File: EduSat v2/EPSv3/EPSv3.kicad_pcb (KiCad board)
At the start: 2 copper layers, 1 part

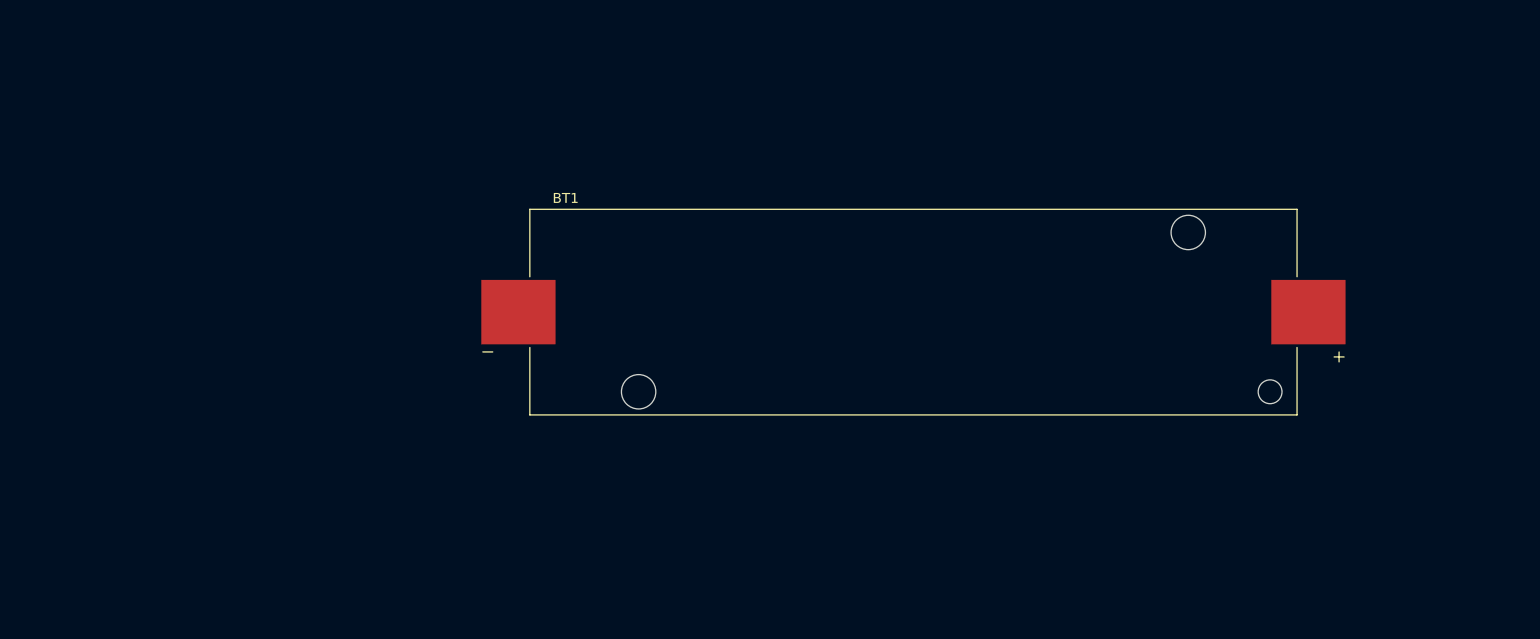
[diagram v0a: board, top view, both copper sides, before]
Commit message: EPS updates
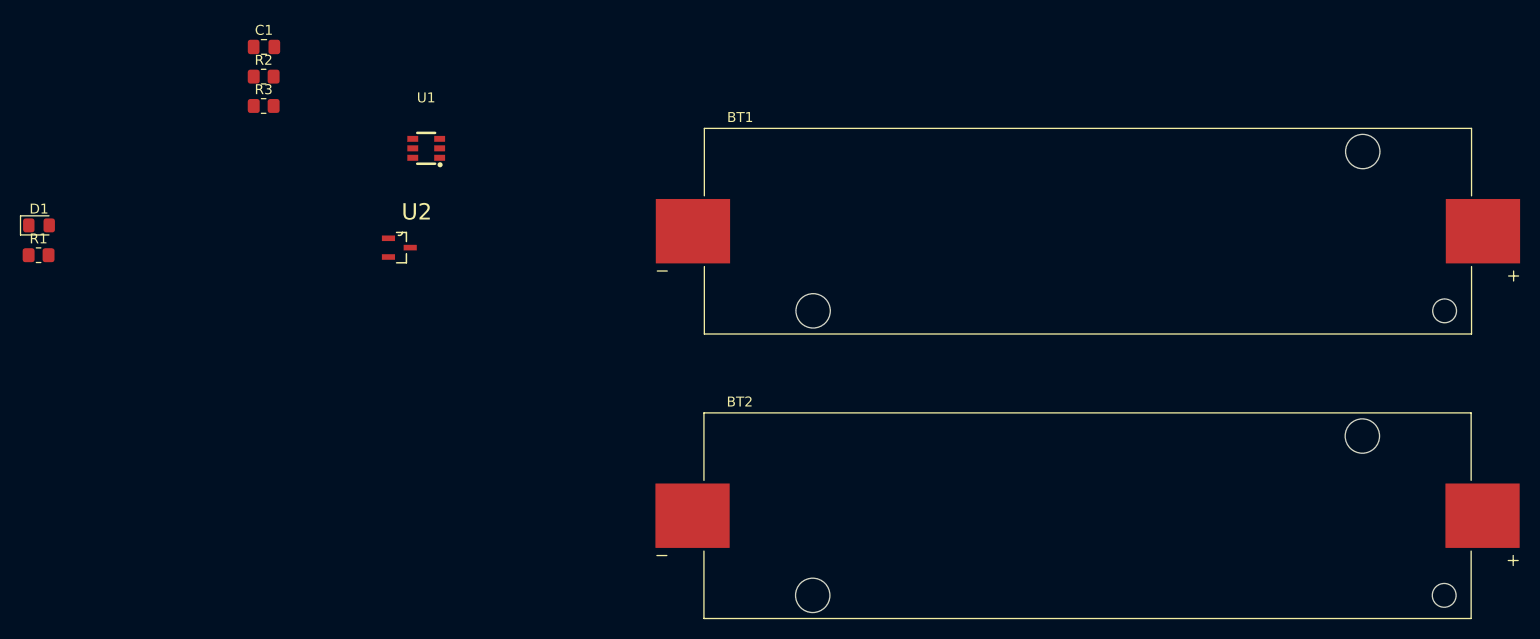
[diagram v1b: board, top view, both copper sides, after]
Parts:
- added BT2: 1042, Battery_Holder_1:BAT_1042, F.Cu at (218.1, 80.0)
- added C1: 0.1uF, Capacitor_SMD:C_0805_2012Metric_Pad1.18x1.45mm_HandSolder, F.Cu at (135.4, 32.9)
- added D1: Yellow LED, LED_SMD:LED_0805_2012Metric_Pad1.15x1.40mm_HandSolder, F.Cu at (112.8, 50.9)
- added R1: 100Ω, Resistor_SMD:R_0805_2012Metric_Pad1.20x1.40mm_HandSolder, F.Cu at (112.8, 53.8)
- added R2: 1kΩ, Resistor_SMD:R_0805_2012Metric_Pad1.20x1.40mm_HandSolder, F.Cu at (135.4, 35.9)
- added R3: 100Ω, Resistor_SMD:R_0805_2012Metric_Pad1.20x1.40mm_HandSolder, F.Cu at (135.4, 38.9)
- added U1: ~, DW06D:SOT-23-6_L2.9-W1.6-P0.95-LS2.8-BR, F.Cu at (151.7, 43.1)
- added U2: IRLML6344TRPBF, IRLML6344TRPBF:SOT95P240X112-3N, F.Cu at (149.0, 53.1)
- BT1: footprint BatteryHolderSingle:BAT_1042 -> Battery_Holder_1:BAT_1042
- moved BT1 19.3 mm to (218.2, 51.4)
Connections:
- BT1 pad N: unconnected-(BT1-PadN) -> Net-(U2-D)
- BT1 pad P: unconnected-(BT1-PadP) -> Net-(D1-K)
